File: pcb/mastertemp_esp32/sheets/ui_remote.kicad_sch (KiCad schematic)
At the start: 0 parts

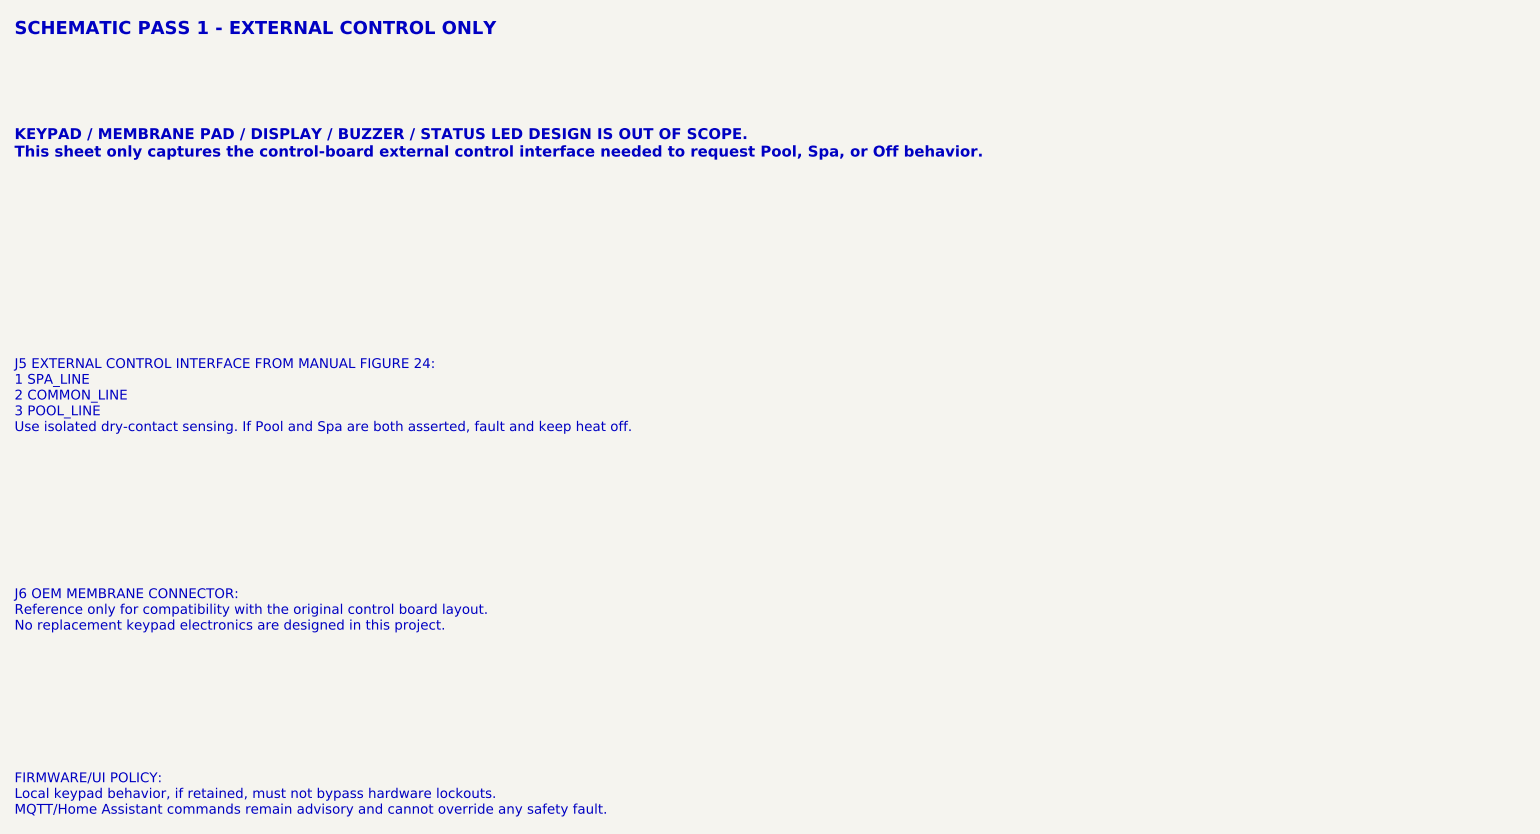
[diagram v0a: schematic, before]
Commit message: AI
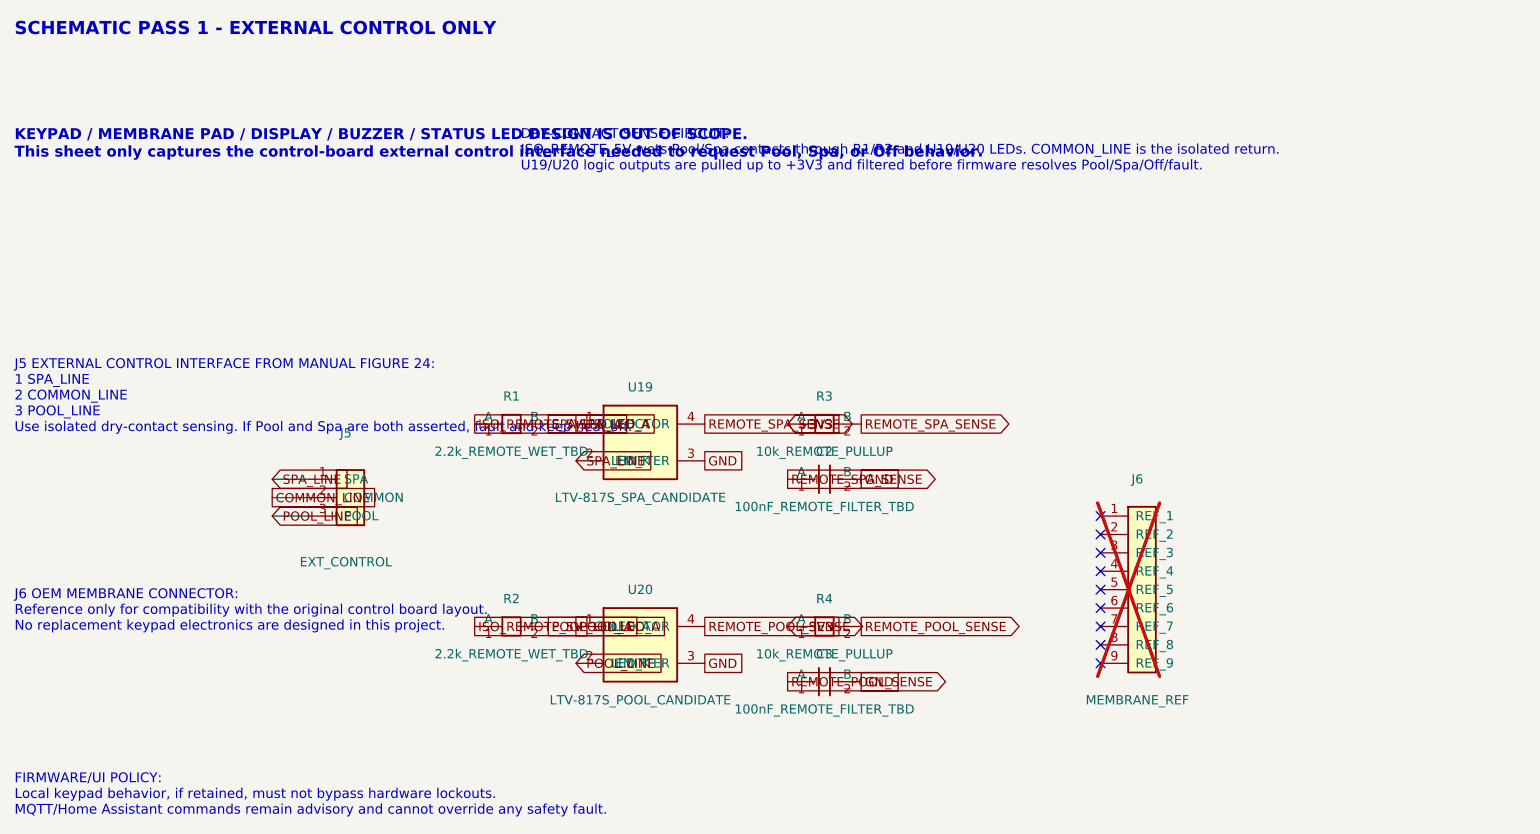
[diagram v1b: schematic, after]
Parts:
- added C2, C3: 100nF_REMOTE_FILTER_TBD, Capacitor_SMD:C_0805_2012Metric, symbol mastertemp_esp32:Capacitor_2pin
- added J5: EXT_CONTROL, Connector_Phoenix_MSTB:PhoenixContact_MSTBA_2,5_3-G-5,08_1x03_P5.08mm_Horizontal, symbol mastertemp_esp32:ExternalControl_3P
- added J6: MEMBRANE_REF, Connector_Phoenix_MSTB:PhoenixContact_MSTBVA_2,5_9-G-5,08_1x09_P5.08mm_Vertical, symbol mastertemp_esp32:MembraneReference_9P
- added R1, R2: 2.2k_REMOTE_WET_TBD, Resistor_SMD:R_0805_2012Metric, symbol mastertemp_esp32:Resistor_2pin
- added R3, R4: 10k_REMOTE_PULLUP, Resistor_SMD:R_0805_2012Metric, symbol mastertemp_esp32:Resistor_2pin
- added U19: LTV-817S_SPA_CANDIDATE, Package_DIP:DIP-4_W7.62mm, symbol mastertemp_esp32:Optocoupler_4pin
- added U20: LTV-817S_POOL_CANDIDATE, Package_DIP:DIP-4_W7.62mm, symbol mastertemp_esp32:Optocoupler_4pin
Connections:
- new net +3V3: R3.1 (A), R4.1 (A)
- new net COMMON_LINE: J5.2 (COMMON)
- new net GND: C2.2 (B), C3.2 (B), U19.3 (EMITTER), U20.3 (EMITTER)
- new net ISO_REMOTE_5V: R1.1 (A), R2.1 (A)
- new net POOL_LED_A: R2.2 (B), U20.1 (LED_A)
- new net POOL_LINE: J5.3 (POOL), U20.2 (LED_K)
- new net REMOTE_POOL_SENSE: C3.1 (A), R4.2 (B), U20.4 (COLLECTOR)
- new net REMOTE_SPA_SENSE: C2.1 (A), R3.2 (B), U19.4 (COLLECTOR)
- new net SPA_LED_A: R1.2 (B), U19.1 (LED_A)
- new net SPA_LINE: J5.1 (SPA), U19.2 (LED_K)
- no-connect marks 0 -> 9
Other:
- note added: "DRY-CONTACT SENSE CIRCUIT: ISO_REMOTE_5V wets Pool/Spa contacts through R1/R2 and U19/U20 LEDs. COMMON_LINE is the isolated return. U19/U20 logic outputs are pulled up to +3V3 and filtered before firmware resolves Pool/Spa/Off/fault."
